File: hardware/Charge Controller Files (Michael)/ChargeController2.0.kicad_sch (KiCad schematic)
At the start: 82 parts, among them J1 Conn_01x02_Pin, J10 Conn-1x2, J11 Conn-1x2, J12 Conn-1x2, J13 Conn-1x2, J14 Conn-1x2, J15 Conn-1x2, J16 Conn-1x2, J17 SCL_MAS_01x01_Pin, J18 SDA_MAS_01x01_Pin, J2 SP_01x02_Pin, J3 SYS-1x2, J4 3.3V_PULLUP_01x01_Pin, J5 BATT_01x02_Pin, J6 Conn-1x2, J7 Conn-1x2, J8 Conn-1x2, J9 Conn-1x2, Q5 AONS66614, Q6 AONS66614, Q7 AONS66614, Q8 AONS66614, U1 BQ25756RRVR

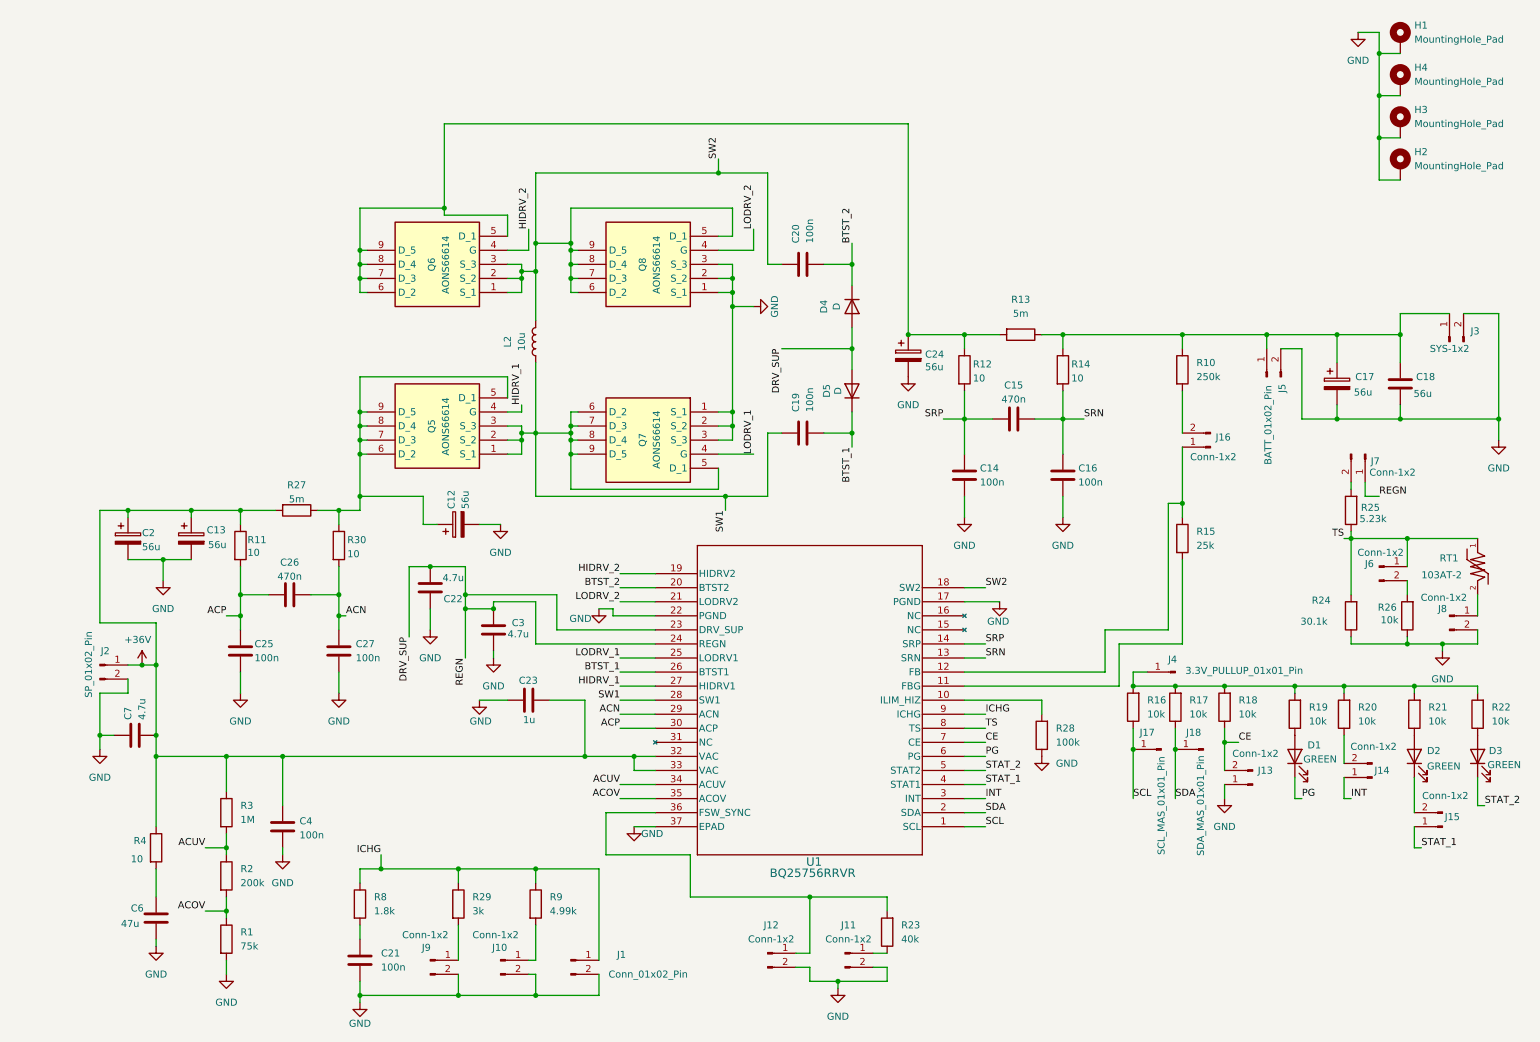
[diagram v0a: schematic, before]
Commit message: Inhibits Draft
Inhibits First Draft - MP
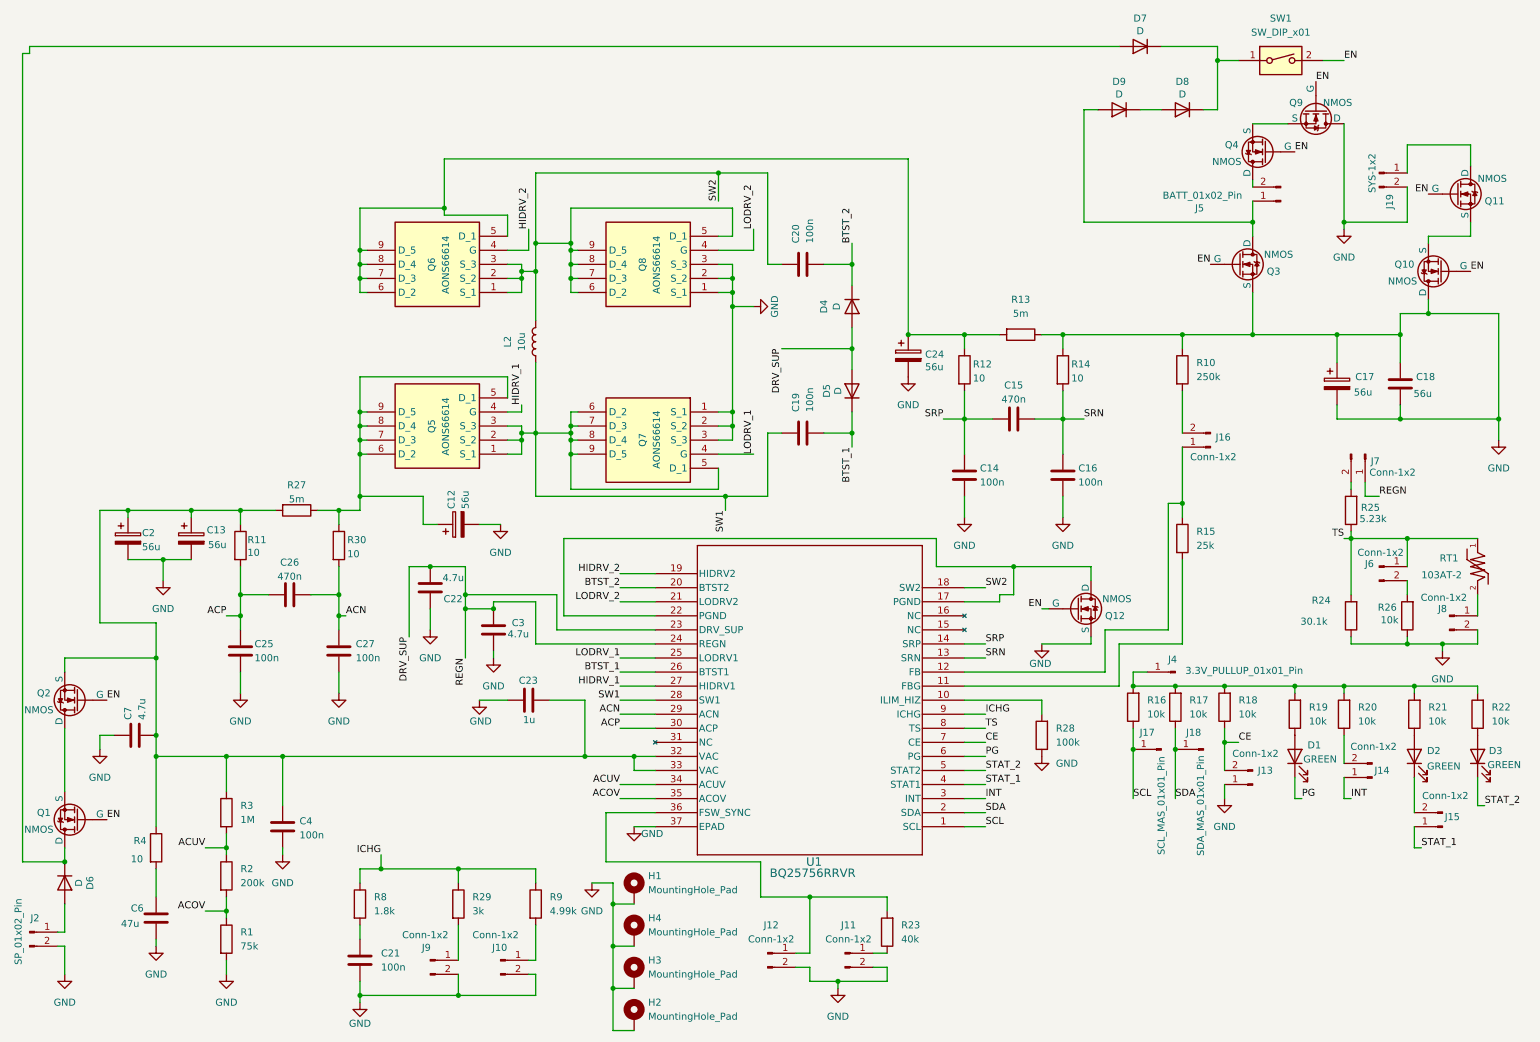
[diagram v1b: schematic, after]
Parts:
- removed J1: Conn_01x02_Pin, symbol Connector:Conn_01x02_Pin
- removed J3: SYS-1x2, Connector_PinSocket_2.54mm:PinSocket_1x02_P2.54mm_Vertical, symbol Connector:Conn_01x02_Pin
- added D6, D7, D8, D9: D, symbol Device:D
- added J19: SYS-1x2, Connector_PinSocket_2.54mm:PinSocket_1x02_P2.54mm_Vertical, symbol Connector:Conn_01x02_Pin
- added Q1, Q10, Q11, Q12, Q2, Q3, Q4, Q9: NMOS, symbol Simulation_SPICE:NMOS
- added SW1: SW_DIP_x01, symbol Switch:SW_DIP_x01
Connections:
- net GND: now also C17.1, C18.1, R10.1, R13.1, R14.1, J19.2 (Pin_2), Q10.1 (D), Q12.3 (S), Q3.3 (S), Q9.1 (D); no longer J5.2 (Pin_2), U1.17 (PGND), U1.22 (PGND)
- net +36V: no longer names the net of C13.1, C2.1, C23.1, C4.1, C7.2, R11.1, R27.2, R3.1, R4.1, U1.32 (VAC), U1.33 (VAC)
- net +36V: now also Q2.3 (S); no longer J2.1 (Pin_1)
- new net: J19.1 (Pin_1), Q11.1 (D)
- new net: Q4.3 (S), Q9.3 (S)
- new net: Q1.3 (S), Q2.1 (D)
- new net: D7.1 (K), D8.1 (K), SW1.1
- new net: D8.2 (A), D9.1 (K)
- new net: D9.2 (A), J5.1 (Pin_1), Q3.1 (D)
- new net: J5.2 (Pin_2), Q4.1 (D)
- new net: D6.1 (K), D7.2 (A), Q1.1 (D)
- new net: Q10.3 (S), Q11.3 (S)
- new net: Q12.1 (D), U1.17 (PGND), U1.22 (PGND)
- new net: D6.2 (A), J2.1 (Pin_1)
- new net EN: Q1.2 (G), Q10.2 (G), Q11.2 (G), Q12.2 (G), Q2.2 (G), Q3.2 (G), Q4.2 (G), Q9.2 (G), SW1.2
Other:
- moved on the sheet: H1, H2, H3, H4, J2, J5
